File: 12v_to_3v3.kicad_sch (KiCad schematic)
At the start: 6 parts, among them U3 ADP1108AR-3.3

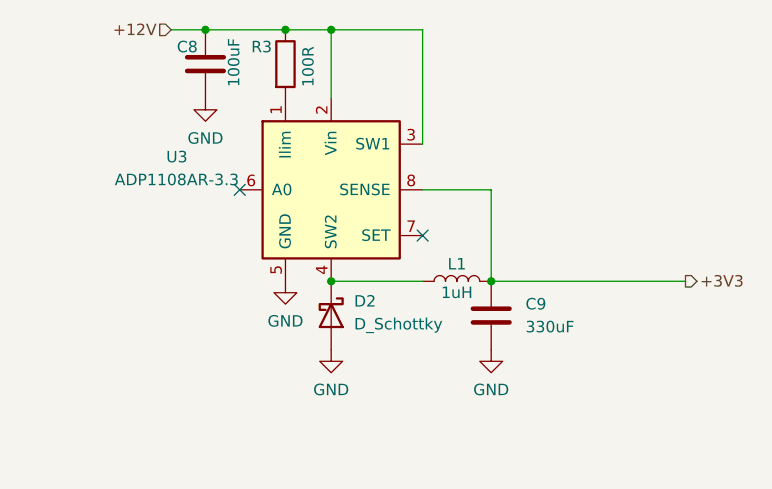
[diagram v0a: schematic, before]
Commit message: Fix PCB
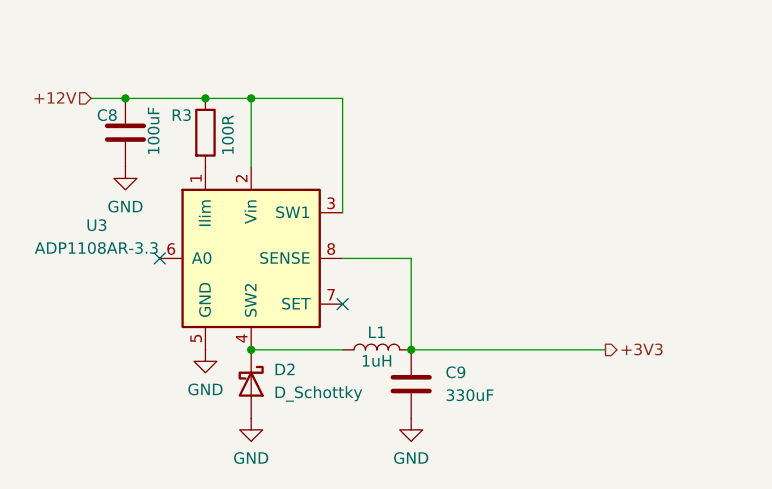
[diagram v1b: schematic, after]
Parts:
- C8: footprint Capacitor_SMD:C_1206_3216Metric -> Capacitor_SMD:C_0603_1608Metric
- C9: footprint Capacitor_SMD:C_0805_2012Metric -> Capacitor_SMD:C_0603_1608Metric
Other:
- moved on the sheet: C8, C9, D2, L1, R3, U3
